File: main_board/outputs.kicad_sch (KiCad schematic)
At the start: 74 parts, among them J10 3.5mm Jack, J11 3.5mm Jack, J12 3.5mm Jack, J13 3.5mm Jack, J14 3.5mm Jack, J15 3.5mm Jack, J8 3.5mm Jack, J9 3.5mm Jack, Q1 MMBT3904, U1 TL072CDR, U15 LM4132xMF-3.3, U2 TL072CDR, U5 TL072CDR, U6 AD5328, U7 L78L05_SOT89, U8 TL072CDR, U9 TL072CDR

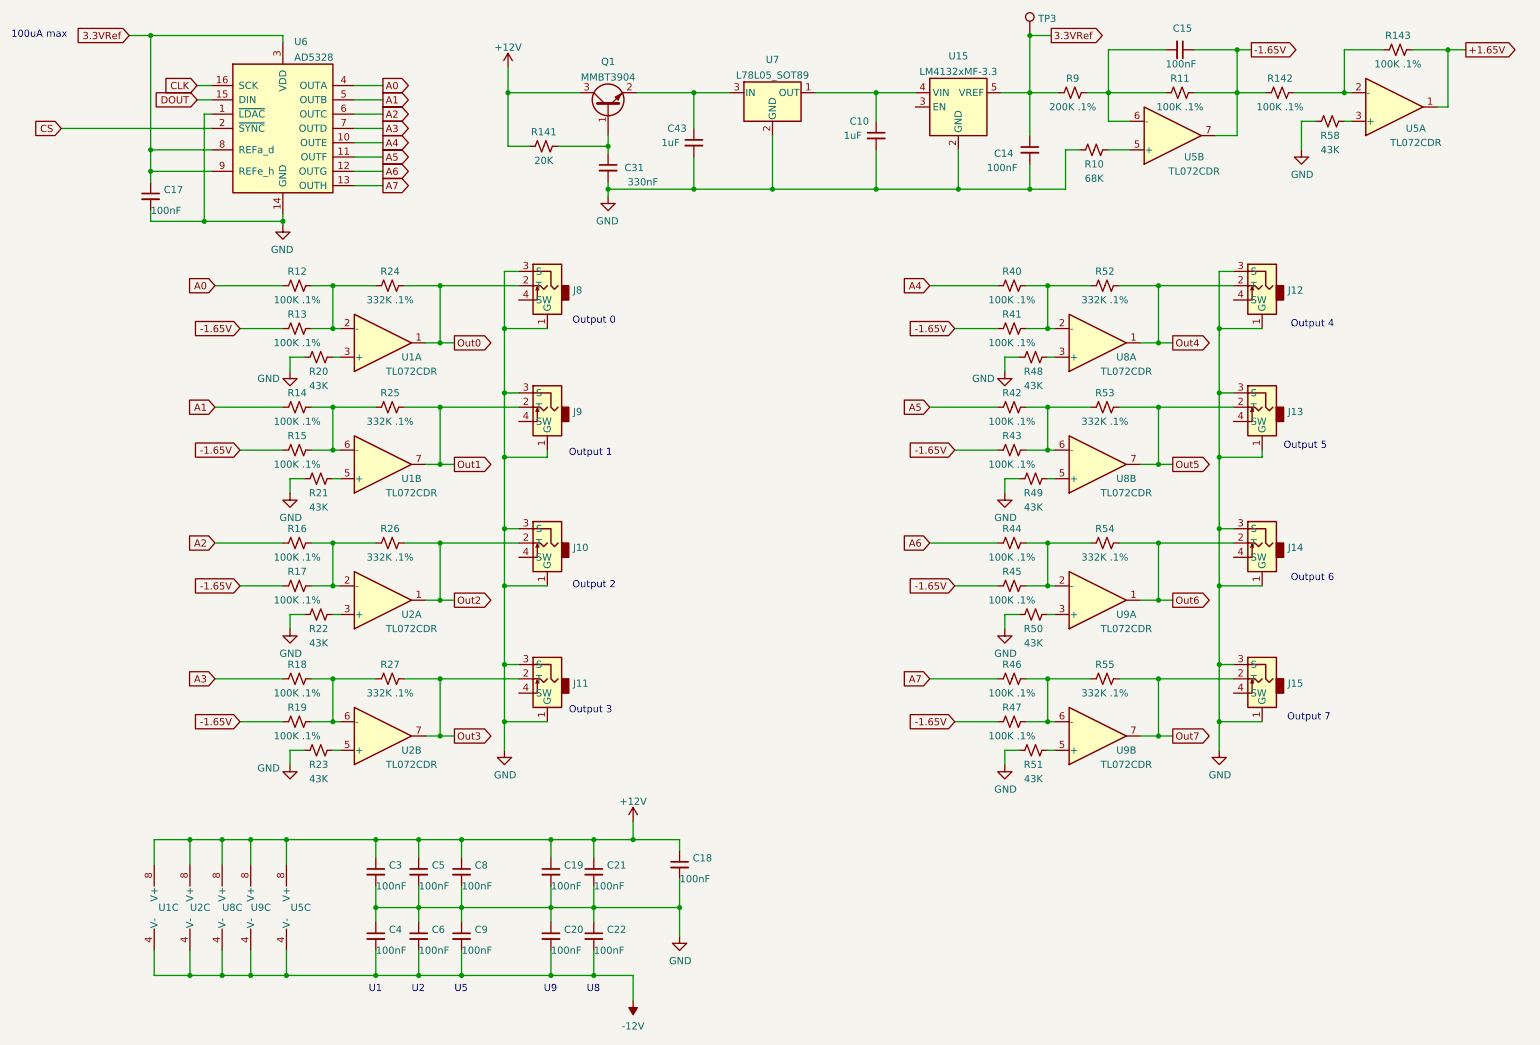
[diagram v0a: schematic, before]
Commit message: Upgrades board to v5. Adds Bonk Daddy.
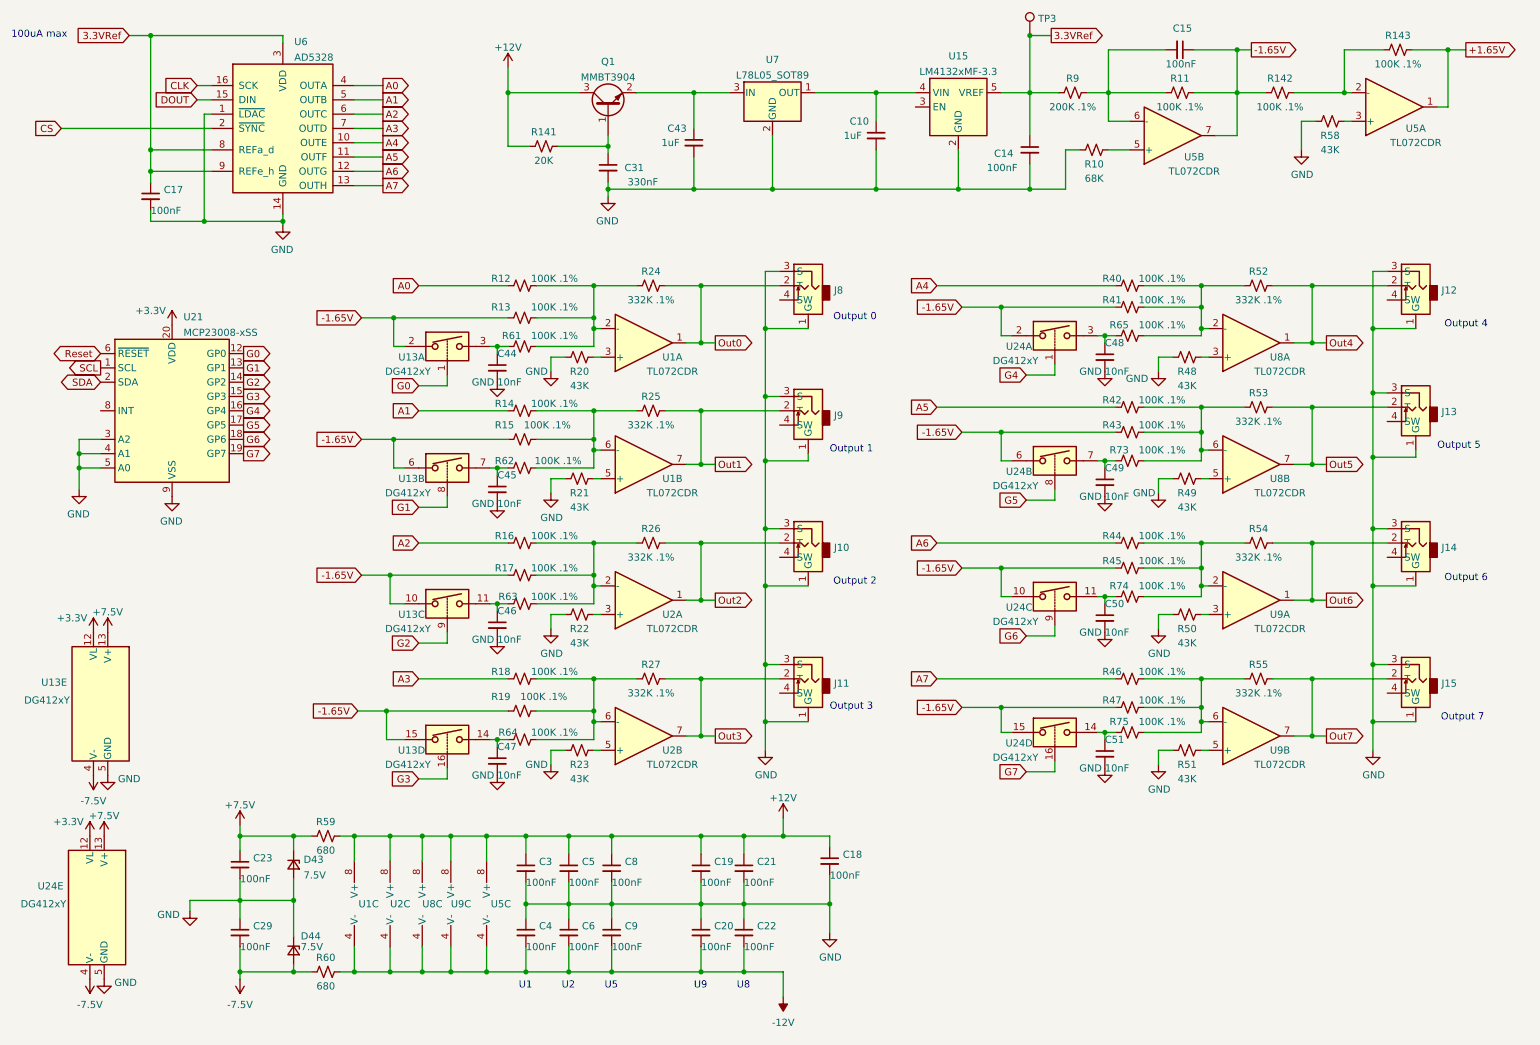
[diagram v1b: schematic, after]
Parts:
- added C23, C29: 100nF, Capacitor_SMD:C_0805_2012Metric_Pad1.18x1.45mm_HandSolder, symbol Device:C_Small
- added C44, C45, C46, C47, C48, C49, C50, C51: 10nF, Capacitor_SMD:C_0805_2012Metric_Pad1.18x1.45mm_HandSolder, symbol Device:C_Small
- added D43, D44: 7.5V, Diode_SMD:D_SOD-123, symbol Device:D_Zener_Small
- added R59, R60: 680, Resistor_SMD:R_0805_2012Metric_Pad1.20x1.40mm_HandSolder, symbol Device:R_Small_US
- added R61, R62, R63, R64, R65, R73, R74, R75: 100K .1%, Resistor_SMD:R_0805_2012Metric_Pad1.20x1.40mm_HandSolder, symbol Device:R_Small_US
- added U13, U24: DG412xY, Package_SO:SOIC-16_3.9x9.9mm_P1.27mm, symbol Analog_Switch:DG412xY
- added U21: MCP23008-xSS, Package_SO:SSOP-20_5.3x7.2mm_P0.65mm, symbol Interface_Expansion:MCP23008-xSS
- TP3: footprint TestPoint:TestPoint_Keystone_5005-5009_Compact -> TestPoint:TestPoint_Keystone_5000-5004_Miniature;  LCSC Part # (none) -> C238123; Digi-Key Part 36-5006-ND -> 36-5002-ND
- U2, U8: footprint Package_SO:SOIC-8-1EP_3.9x4.9mm_P1.27mm_EP2.29x3mm -> Package_SO:SOIC-8_3.9x4.9mm_P1.27mm
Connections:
- net +12V: now also R59.1
- net -1.65V: now also U13.10, U13.15, U13.2, U13.6, U24.10, U24.15, U24.2, U24.6
- net -12V: now also R60.1
- net GND: now also C23.2, C29.1, C44.2, C45.2, C46.2, C47.2, C48.2, C49.2, C50.2, C51.2, D43.2 (A), D44.1 (K), U13.5 (GND), U21.3 (A2), U21.4 (A1), U21.5 (A0), U21.9 (VSS), U24.5 (GND)
- net at R12.1, R13.1, R24.2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: now also R61.1
- net at R46.1, R47.1, R55.2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: now also R75.1
- net at R14.1, R15.1, R25.2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: now also R62.1
- net at R42.1, R43.1, R53.2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: now also R73.1
- net at R16.1, R17.1, R26.2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: now also R63.1
- net at R44.1, R45.1, R54.2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: now also R74.1
- net at R18.1, R19.1, R27.2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: now also R64.1
- net at R40.1, R41.1, R52.2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: now also R65.1
- new net: C48.1, R65.2, U24.3
- new net: C50.1, R74.2, U24.11
- new net: C46.1, R63.2, U13.11
- new net: C45.1, R62.2, U13.7
- new net: C44.1, R61.2, U13.3
- new net: C47.1, R64.2, U13.14
- new net: C51.1, R75.2, U24.14
- new net: C49.1, R73.2, U24.7
- new net +3V3: U13.12 (VL), U21.20 (VDD), U24.12 (VL)
- new net +7.5V: C23.1, D43.1 (K), R59.2, U13.13 (V+), U24.13 (V+)
- new net -7.5V: C29.2, D44.2 (A), R60.2, U13.4 (V-), U24.4 (V-)
- new net G0: U13.1, U21.12 (GP0)
- new net G1: U13.8, U21.13 (GP1)
- new net G2: U13.9, U21.14 (GP2)
- new net G3: U13.16, U21.15 (GP3)
- new net G4: U21.16 (GP4), U24.1
- new net G5: U21.17 (GP5), U24.8
- new net G6: U21.18 (GP6), U24.9
- new net G7: U21.19 (GP7), U24.16
- new net Reset: U21.6 (~{RESET})
- new net SCL: U21.1 (SCL)
- new net SDA: U21.2 (SDA)
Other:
- moved on the sheet: C18, C19, C20, C21, C22, C3, C4, C5, C6, C8, C9, J10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
